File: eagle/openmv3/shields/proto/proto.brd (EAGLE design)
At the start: 35.6 x 26.7 mm, 2 parts

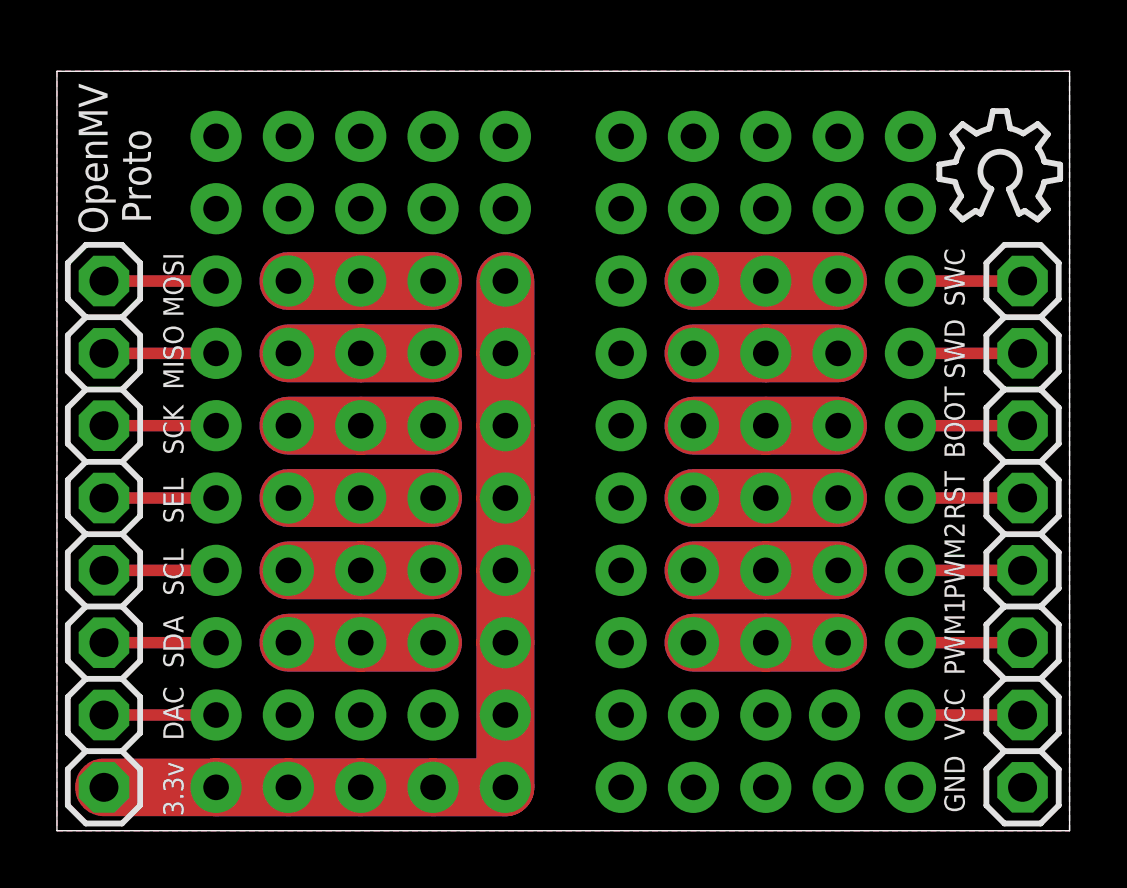
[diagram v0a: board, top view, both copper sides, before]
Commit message: Update design files
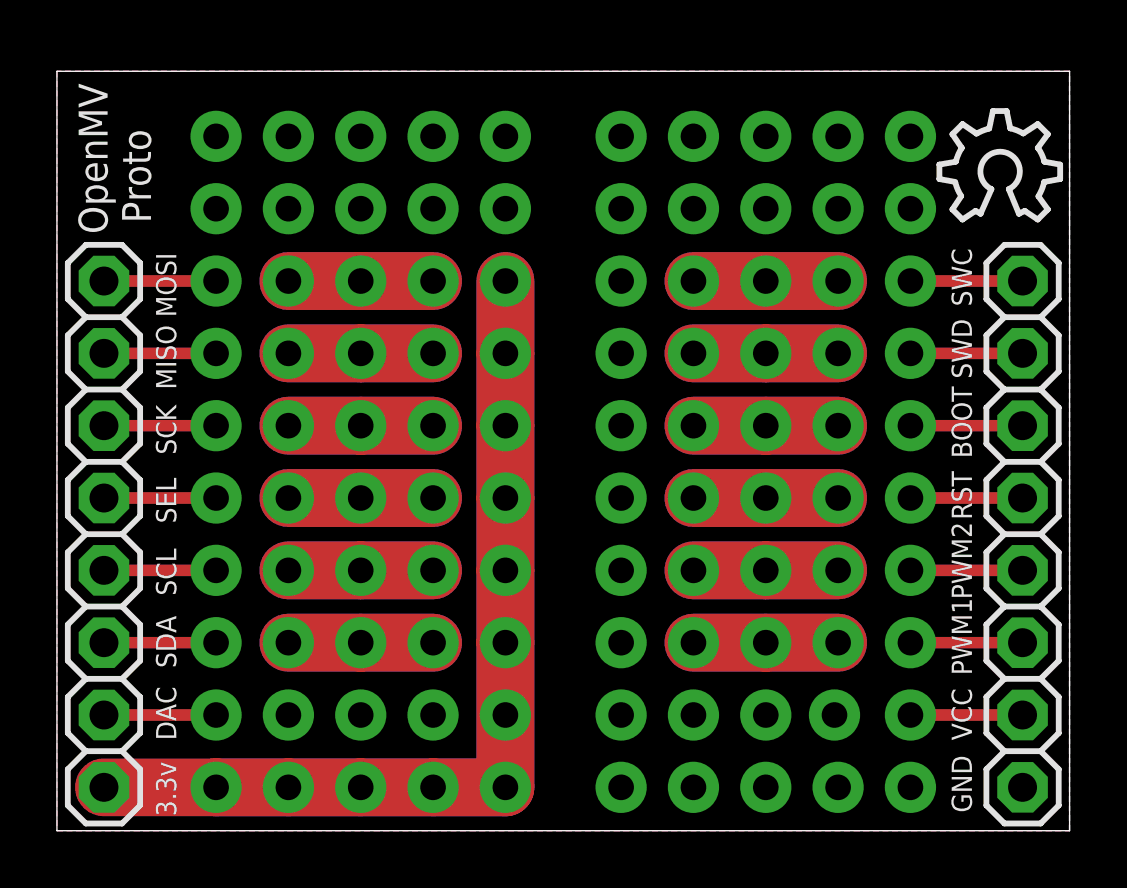
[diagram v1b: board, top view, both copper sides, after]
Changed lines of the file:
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@@
 <text x="38.7477" y="23.495" size="0.8128" layer="48">er is 3.66</text>
 <text x="38.7477" y="33.655" size="0.8128" layer="48">Stackup:</text>
-<text x="4.445" y="3.175" size="0.7112" layer="21" font="vector" ratio="20" rot="R90">DAC</text>
-<text x="4.445" y="8.255" size="0.7112" layer="21" font="vector" ratio="20" rot="R90">SCL</text>
-<text x="4.445" y="5.715" size="0.7112" layer="21" font="vector" ratio="20" rot="R90">SDA</text>
-<text x="4.445" y="10.795" size="0.7112" layer="21" font="vector" ratio="20" rot="R90">SEL</text>
-<text x="4.445" y="13.208" size="0.7112" layer="21" font="vector" ratio="20" rot="R90">SCK</text>
-<text x="4.445" y="15.494" size="0.7112" layer="21" font="vector" ratio="20" rot="R90">MISO</text>
-<text x="31.877" y="15.875" size="0.7112" layer="21" font="vector" ratio="20" rot="R90">SWD</text>
-<text x="31.877" y="18.415" size="0.7112" layer="21" font="vector" ratio="20" rot="R90">SWC</text>
-<text x="31.877" y="13.081" size="0.7112" layer="21" font="vector" ratio="20" rot="R90">BOOT</text>
-<text x="31.877" y="10.922" size="0.7112" layer="21" font="vector" ratio="20" rot="R90">RST</text>
-<text x="31.877" y="5.461" size="0.7112" layer="21" font="vector" ratio="20" rot="R90">PWM1</text>
-<text x="31.877" y="0.635" size="0.7112" layer="21" font="vector" ratio="20" rot="R90">GND</text>
-<text x="4.445" y="0.508" size="0.7112" layer="21" font="vector" ratio="20" rot="R90">3.3v</text>
-<text x="31.877" y="3.175" size="0.7112" layer="21" font="vector" ratio="20" rot="R90">VCC</text>
-<text x="31.877" y="8.128" size="0.7112" layer="21" font="vector" ratio="20" rot="R90">PWM2</text>
-<text x="4.445" y="18.034" size="0.7112" layer="21" font="vector" ratio="20" rot="R90">MOSI</text>
+<text x="4.191" y="3.175" size="0.7112" layer="21" font="vector" ratio="20" rot="R90">DAC</text>
+<text x="4.191" y="8.255" size="0.7112" layer="21" font="vector" ratio="20" rot="R90">SCL</text>
+<text x="4.191" y="5.715" size="0.7112" layer="21" font="vector" ratio="20" rot="R90">SDA</text>
+<text x="4.191" y="10.795" size="0.7112" layer="21" font="vector" ratio="20" rot="R90">SEL</text>
+<text x="4.191" y="13.208" size="0.7112" layer="21" font="vector" ratio="20" rot="R90">SCK</text>
+<text x="4.191" y="15.494" size="0.7112" layer="21" font="vector" ratio="20" rot="R90">MISO</text>
+<text x="32.131" y="15.875" size="0.7112" layer="21" font="vector" ratio="20" rot="R90">SWD</text>
+<text x="32.131" y="18.415" size="0.7112" layer="21" font="vector" ratio="20" rot="R90">SWC</text>
+<text x="32.131" y="13.081" size="0.7112" layer="21" font="vector" ratio="20" rot="R90">BOOT</text>
+<text x="32.131" y="10.922" size="0.7112" layer="21" font="vector" ratio="20" rot="R90">RST</text>
+<text x="32.131" y="5.461" size="0.7112" layer="21" font="vector" ratio="20" rot="R90">PWM1</text>
+<text x="32.131" y="0.635" size="0.7112" layer="21" font="vector" ratio="20" rot="R90">GND</text>
+<text x="4.191" y="0.508" size="0.7112" layer="21" font="vector" ratio="20" rot="R90">3.3v</text>
+<text x="32.131" y="3.175" size="0.7112" layer="21" font="vector" ratio="20" rot="R90">VCC</text>
+<text x="32.131" y="8.128" size="0.7112" layer="21" font="vector" ratio="20" rot="R90">PWM2</text>
+<text x="4.191" y="18.034" size="0.7112" layer="21" font="vector" ratio="20" rot="R90">MOSI</text>
 <text x="1.778" y="20.955" size="1.016" layer="21" font="vector" ratio="22" rot="R90">OpenMV</text>
 <wire x1="13.208" y1="19.304" x2="8.128" y2="19.304" width="2.032" layer="29"/>
@@
 <wire x1="10.668" y1="1.524" x2="13.208" y2="1.524" width="2.032" layer="1"/>
 <wire x1="13.208" y1="1.524" x2="15.748" y2="1.524" width="2.032" layer="1"/>
+<via x="15.748" y="4.064" extent="1-16" drill="0.9" shape="octagon"/>
 <wire x1="15.748" y1="1.524" x2="5.588" y2="1.524" width="2.032" layer="16"/>
-<via x="15.748" y="4.064" extent="1-16" drill="0.9" shape="octagon"/>
 </signal>
 <signal name="N$1">
